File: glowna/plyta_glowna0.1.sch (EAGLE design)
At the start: 223 parts, among them IC1 4504D, IC2 MAX481CSA, IC3 4504D, IC4 OPA4658UU, Q1 CSM-7X-DU, Q2 N-HEXFET-2D_SOT232-IRLL014N, Q3 N-HEXFET-2D_SOT232-IRLL014N, Q4 N-HEXFET-2D_SOT232-IRLL014N, Q5 N-HEXFET-2D_SOT232-IRLL014N, Q6 N-HEXFET-2D_SOT232-IRLL014N, X1 MINI-USB_SHIELD5P2-32005-601

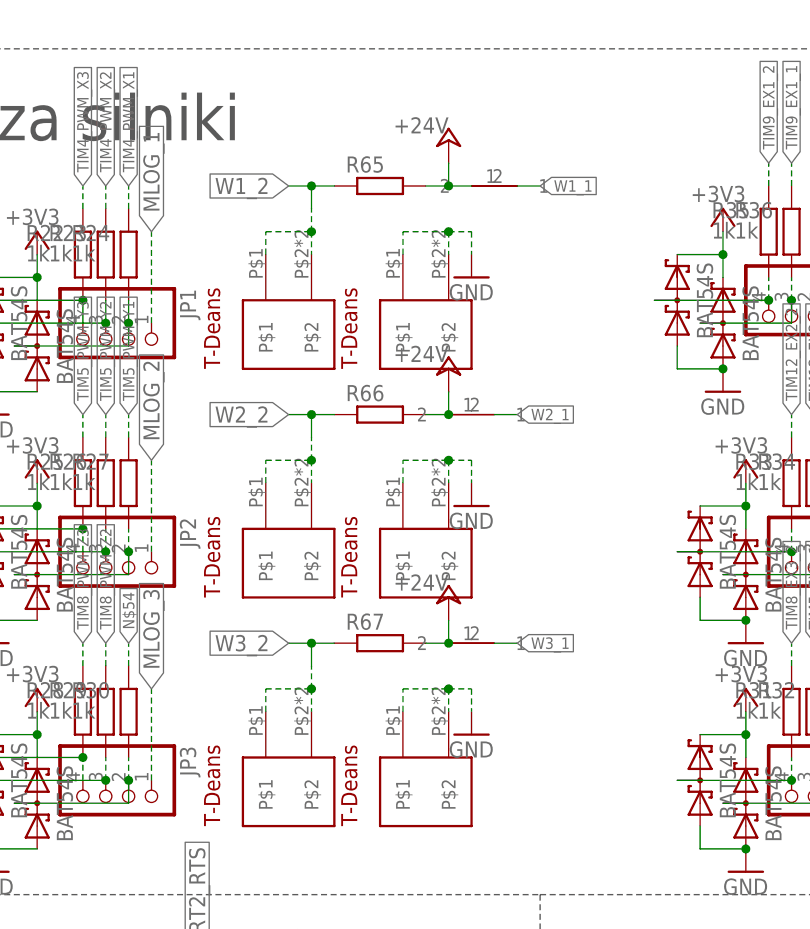
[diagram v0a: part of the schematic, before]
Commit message: to juz jest koniec
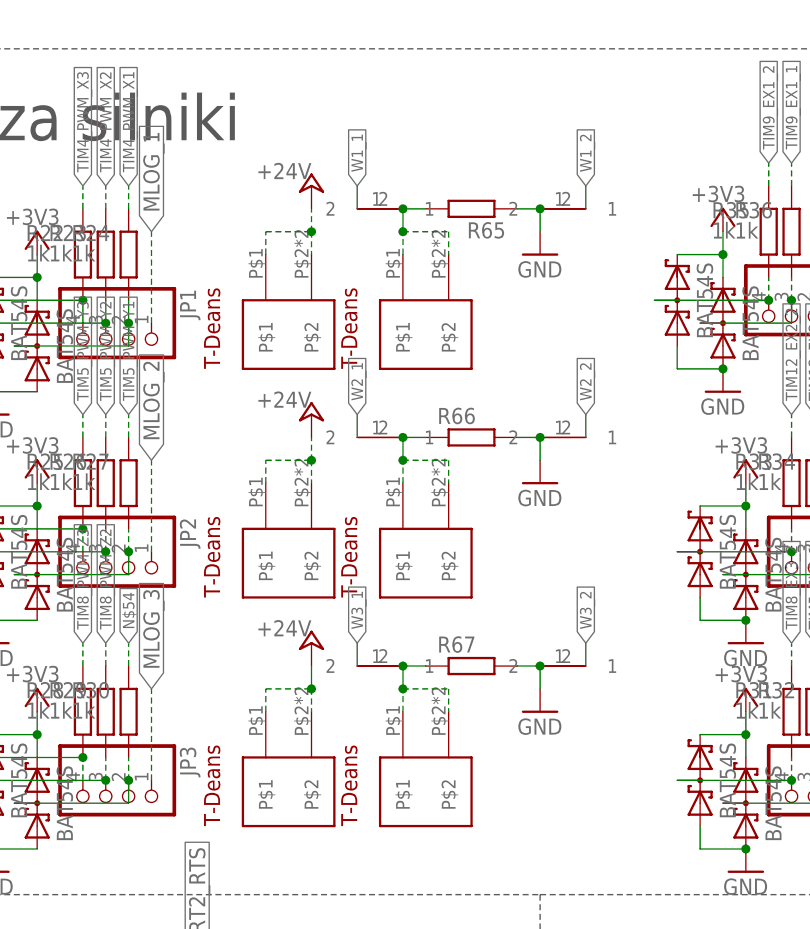
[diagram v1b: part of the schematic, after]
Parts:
- added U$23, U$24, U$25: SEPARATOR, robione:SEPARATOR
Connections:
- new net N$77: R65.2, U$23.2, U$8.P$1, U$8.P$2
- new net N$78: R66.1, U$10.P$1, U$10.P$2, U$24.2
- new net N$83: R67.1, U$12.P$1, U$12.P$2, U$25.2
- net +24V: now also U$11.P$1, U$11.P$2, U$7.P$1, U$7.P$2, U$9.P$1, U$9.P$2; no longer R65.2, R66.2, R67.2, U$20.1, U$21.1, U$22.1
- net GND: now also R65.1, R66.2, R67.2, U$20.1, U$21.1, U$22.1; no longer U$10.P$1, U$10.P$2, U$12.P$1, U$12.P$2, U$8.P$1, U$8.P$2
- net W1_1: now also U$23.1; no longer U$20.2
- net W1_2: now also U$20.2; no longer R65.1, U$7.P$1, U$7.P$2
- net W2_1: now also U$24.1; no longer U$21.2
- net W2_2: now also U$21.2; no longer R66.1, U$9.P$1, U$9.P$2
- net W3_1: now also U$25.1; no longer U$22.2
- net W3_2: now also U$22.2; no longer R67.1, U$11.P$1, U$11.P$2
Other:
- moved on the sheet: R65, R66, R67
